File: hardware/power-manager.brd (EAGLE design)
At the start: 74 x 34 mm, 77 parts, among them IC1 ATMEGA168-AU, K1 G6J-2FL-Y, K2 G6J-2FL-Y, K3 G6J-2FL-Y, Q1 BSS138, Q2 BSS138, Q3 BSS138, U1 V_REG_LDOSMD, U2 INA219, U3 TPS2552, U6 INA219, U7 TPS2552, U8 INA219, X2 MC2, X3 MC2, Y1 12MHz

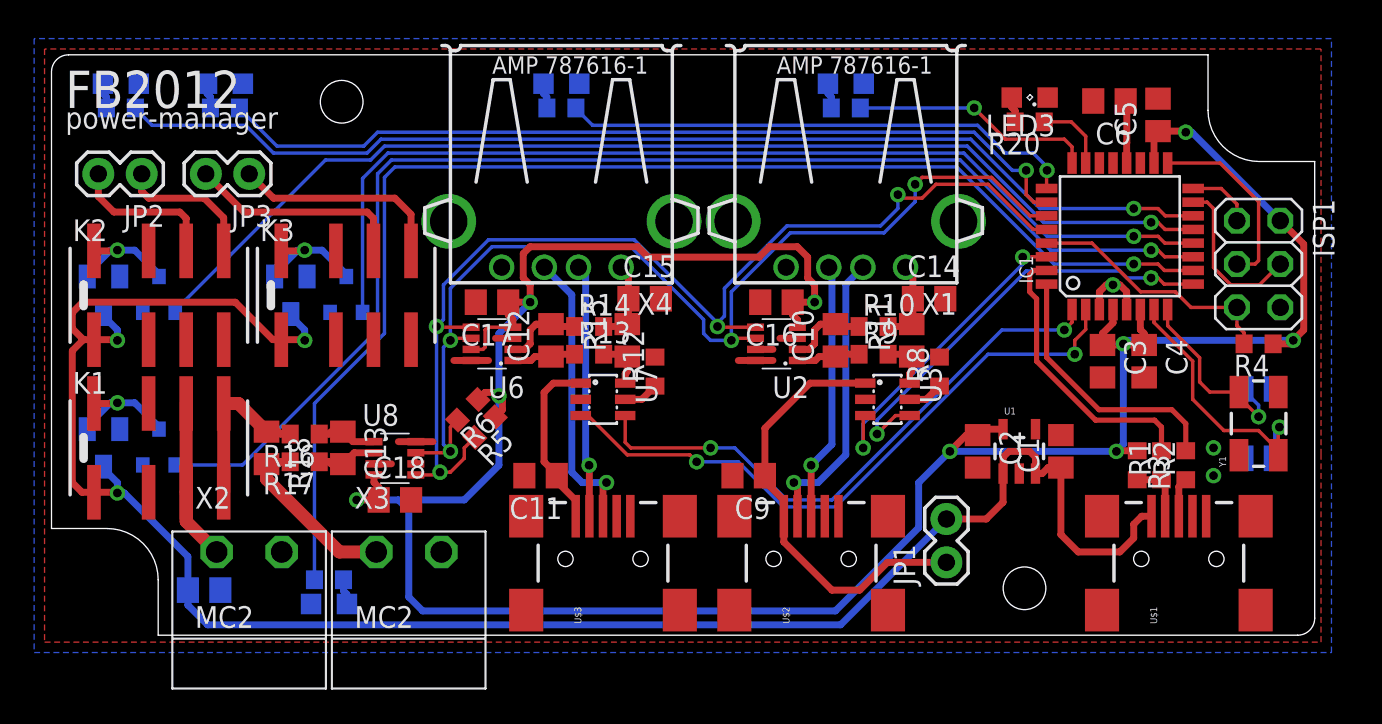
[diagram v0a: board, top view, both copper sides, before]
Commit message: hw: rc2
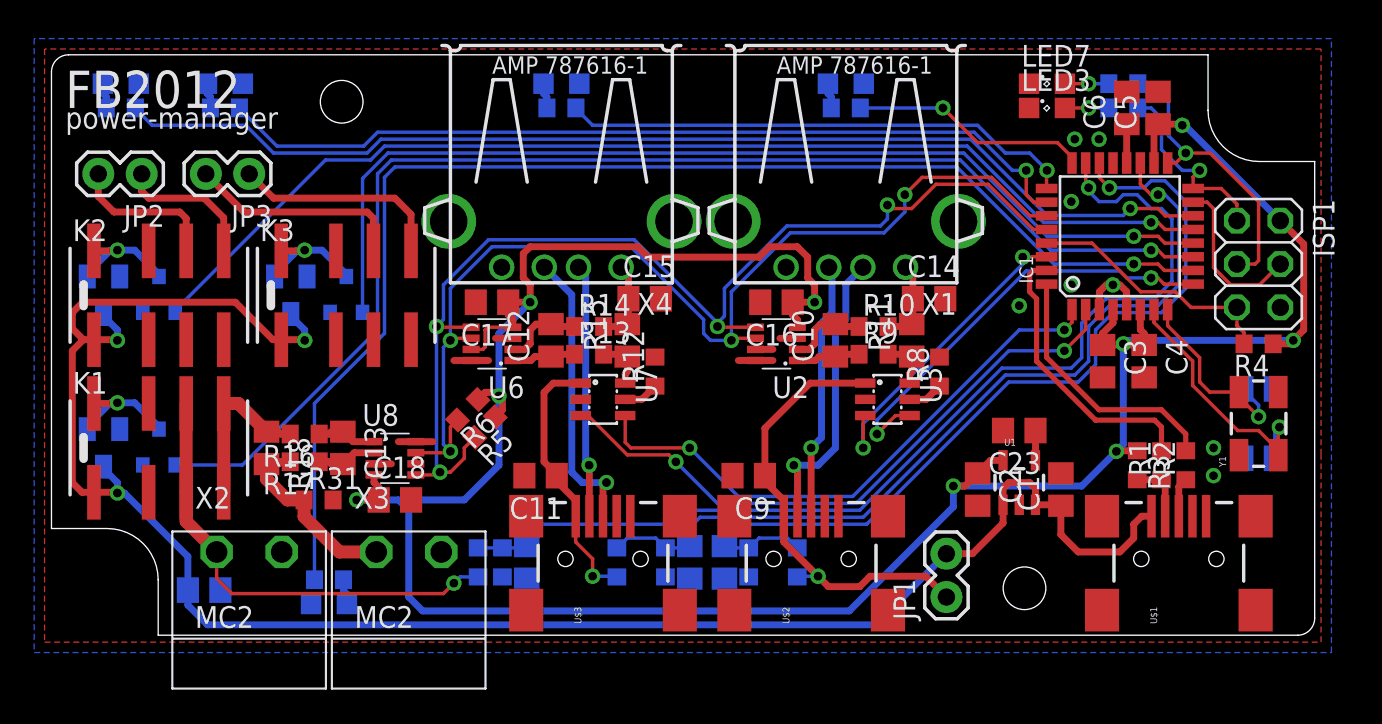
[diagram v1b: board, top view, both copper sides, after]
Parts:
- added C20, C21, C22, C23: .1u, rcl:C0805
- added LED7: (no value), led:SML0805
- added R24, R25, R26, R27, R28, R29: 10k, rcl:R0603
- added R30: 330, rcl:R0603
- added R31: 100k, rcl:R0603
- U1: value V_REG_LDOSMD -> MIC5301
- moved R20 5.55 mm to (62.8, 30.9), flipped to the bottom, turned to 0 degrees
- moved C1 2.24 mm to (59.1, 8.53)
- moved C2 2.24 mm to (54.3, 8.53)
- moved JP1 2.03 mm to (52.4, 2.24)
- moved U1 1.83 mm to (56.7, 8.94)
- moved LED3 1.18 mm to (58.3, 30.9), turned to 0 degrees
- moved C6 1.09 mm to (63.0, 30.9), turned to 90 degrees
- moved C5 0.41 mm to (64.8, 30.9)
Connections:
- removed net LED_SYS: IC1.23, R20.1
- removed net N$21: K1.3, K1.6, X2.1
- new net POWER_ADC: C22.1, IC1.23, R28.2, R29.1
- new net POWER_IN: K1.3, K1.6, R28.1, X2.1
- new net USB1_ADC: C20.1, IC1.22, R24.2, R25.1
- new net USB1_IN: C9.1, JP1.1, R24.1, U$2.VBUS, U3.1
- new net USB2_ADC: C21.1, IC1.19, R26.2, R27.1
- new net USB2_IN: C11.1, R26.1, U$3.VBUS, U7.1
- net GND: now also C20.2, C21.2, C22.2, C23.2, LED7.C, R25.2, R27.2, R29.2, R31.2
- net MISO: now also R20.1
- net N$10: now also LED7.A, R30.2; no longer C11.1, U$3.VBUS, U7.1
- net N$19: now also R31.1
- net N$5: now also C23.1, U1.4; no longer C9.1, JP1.1, U$2.VBUS, U3.1
- net SCK: now also R30.1
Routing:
- net POWER_ADC: track 0.00 -> 60.1 mm, vias 0 -> 1
- net USB1_ADC: track 0.00 -> 51.7 mm, vias 0 -> 1
- net USB2_ADC: track 0.00 -> 50.1 mm, vias 0 -> 1
- net POWER_IN: track 0.00 -> 27.1 mm, vias 0 -> 1
- net USB1_IN: track 0.00 -> 26.7 mm, vias 0 -> 1
- net N$5: track 25.5 -> 1.75 mm
- net USB2_IN: track 0.00 -> 15.8 mm, vias 0 -> 1
- net N$21: track 9.44 -> 0.00 mm
- net N$10: track 10.4 -> 2.57 mm, vias 0 -> 1
- net MISO: track 3.91 -> 11.3 mm, vias 0 -> 1
- net SCK: track 11.1 -> 17.2 mm, vias 0 -> 1
- net LED_SYS: track 4.35 -> 0.00 mm
- net +5V: track 114.0 -> 110.5 mm
- net N$2: track 3.66 -> 2.28 mm
- net N$30: track 1.51 -> 2.57 mm, vias 0 -> 1
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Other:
- board text removed: "www.fabiobaltieri.com"

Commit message: hw: rc3
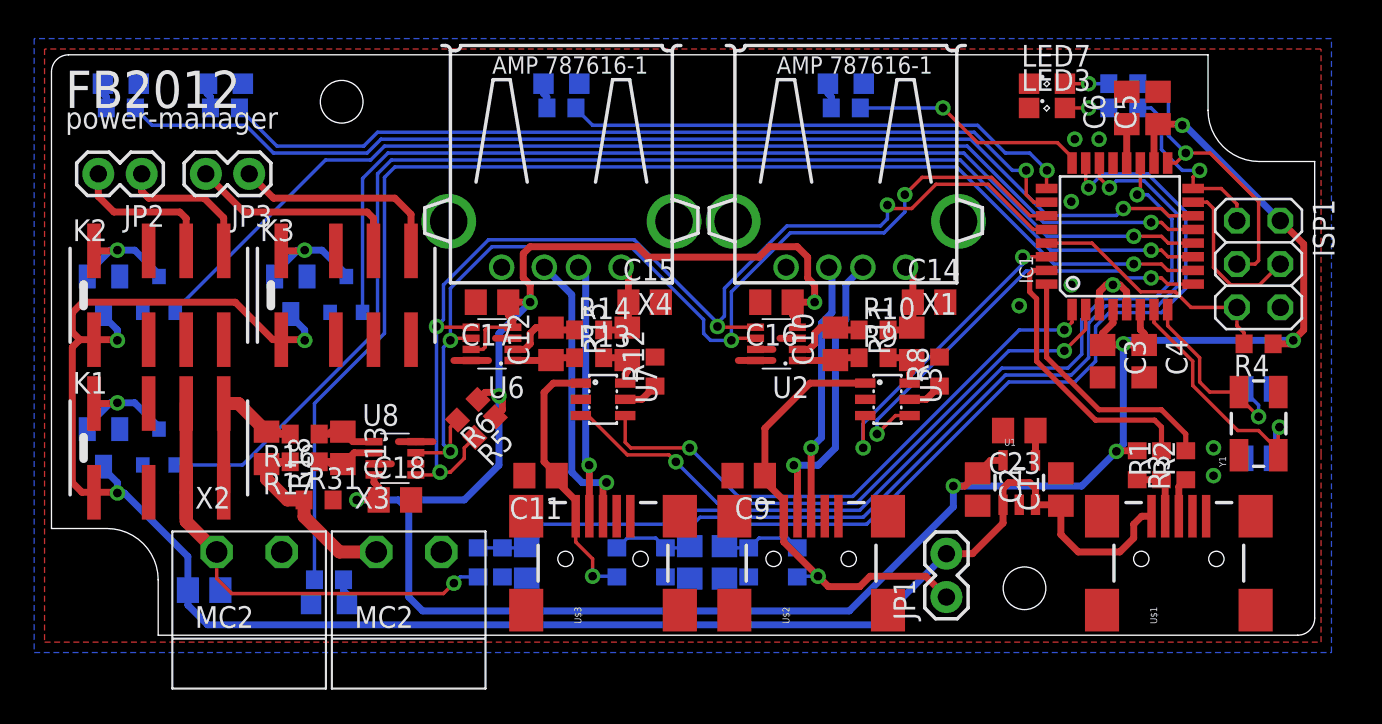
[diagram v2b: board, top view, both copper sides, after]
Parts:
- moved R10 0.20 mm to (48.2, 17.9)
- moved R14 0.20 mm to (31.5, 17.9)
- moved C10 0.20 mm to (45.9, 17.1)
- moved C12 0.20 mm to (29.3, 17.1)
- moved C14 0.20 mm to (51.4, 19.5)
- moved C15 0.20 mm to (34.7, 19.5)
- moved R11 0.20 mm to (50.4, 17.1)
- moved R13 0.20 mm to (31.5, 16.3)
- moved R15 0.20 mm to (33.7, 17.1)
- moved R9 0.20 mm to (48.2, 16.3)
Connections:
- net POWER_ADC: now also IC1.19; no longer IC1.23
- net USB1_ADC: now also IC1.23; no longer IC1.22
- net USB2_ADC: now also IC1.22; no longer IC1.19
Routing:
- net POWER_ADC: track 60.1 -> 57.0 mm
- net USB2_ADC: track 50.1 -> 52.4 mm
- net USB1_ADC: track 51.7 -> 52.7 mm
